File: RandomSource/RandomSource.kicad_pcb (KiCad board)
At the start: 2 copper layers, 154 x 128.5 mm, 74 parts, among them J1 Conn_01x20_Pin, J2 Conn_01x06_Pin, J6 Conn_01x20_Pin, Q1 BC547, Q2 BC547, Q3 BC547, Q4 BC557, Q5 MMBFJ113, Q6 2N7000, U1 TL074, U10 Aux_flush, U11 Aux_flush, U13 Aux_flush, U14 Aux_flush, U2 Aux_flush, U3 Switch, U4 TL074, U5 Switch, U6 Aux_flush, U7 Switch, U8 Switch, U9 Aux_flush

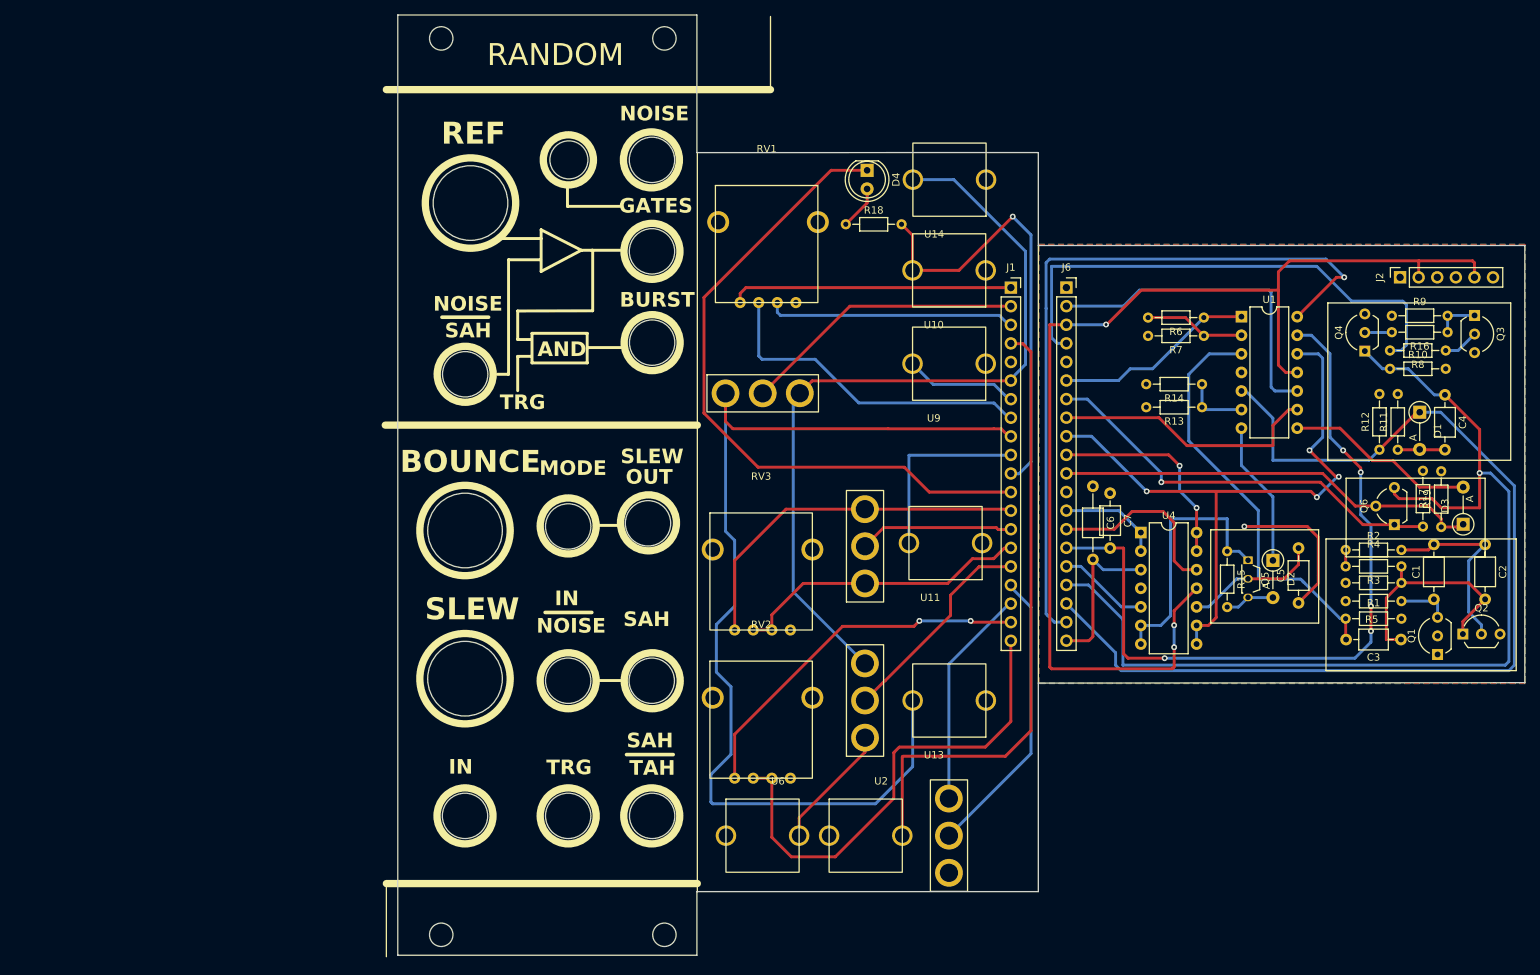
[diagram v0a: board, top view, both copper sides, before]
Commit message: Add files via upload
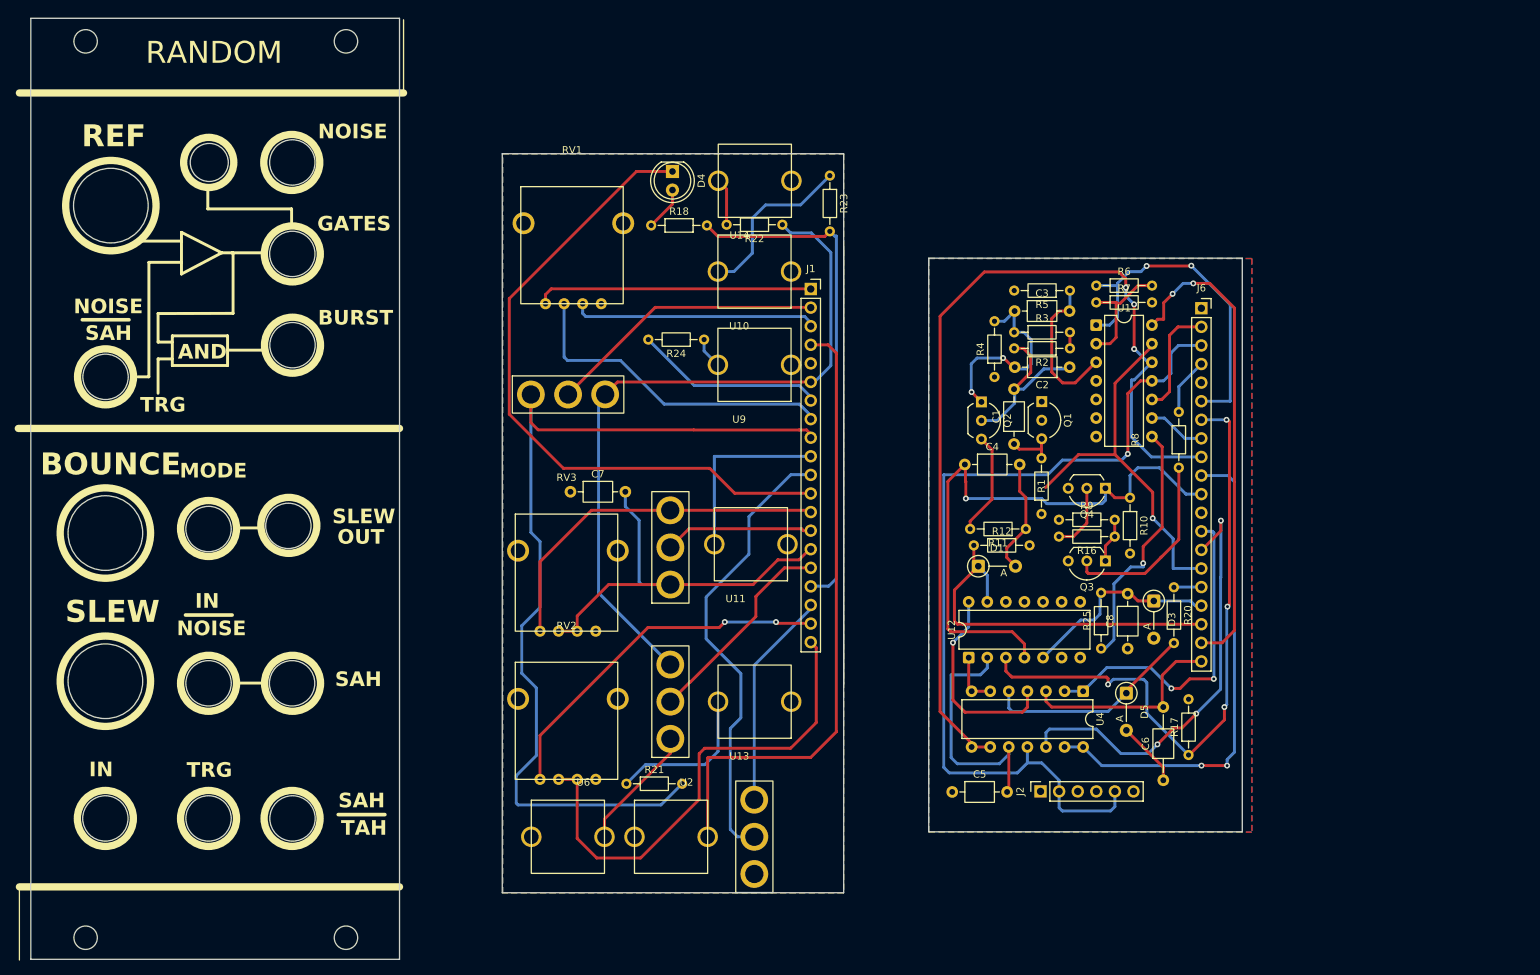
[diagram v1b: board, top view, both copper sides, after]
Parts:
- removed D2: D, Diode_THT:D_A-405_P5.08mm_Vertical_AnodeUp
- removed Q5: MMBFJ113, Package_TO_SOT_THT:TO-92S_Wide
- removed Q6: 2N7000, Package_TO_SOT_THT:TO-92L_Wide
- removed R13: 1k, Resistor_THT:R_Axial_DIN0204_L3.6mm_D1.6mm_P7.62mm_Horizontal
- removed R14, R19: 100k, Resistor_THT:R_Axial_DIN0204_L3.6mm_D1.6mm_P7.62mm_Horizontal
- removed R15: 1M, Resistor_THT:R_Axial_DIN0204_L3.6mm_D1.6mm_P7.62mm_Horizontal
- added C8: 100n, Capacitor_THT:C_Axial_L3.8mm_D2.6mm_P7.50mm_Horizontal, F.Cu at (185.0, 115.1)
- added D5: D, Diode_THT:D_A-405_P5.08mm_Vertical_AnodeUp, F.Cu at (184.8, 121.2)
- added R20: 10k, Resistor_THT:R_Axial_DIN0204_L3.6mm_D1.6mm_P7.62mm_Horizontal, F.Cu at (191.3, 106.7)
- added R21: 1k, Resistor_THT:R_Axial_DIN0204_L3.6mm_D1.6mm_P7.62mm_Horizontal, F.Cu at (116.5, 133.6)
- added R22: 1k, Resistor_THT:R_Axial_DIN0204_L3.6mm_D1.6mm_P7.62mm_Horizontal, F.Cu at (137.8, 57.2)
- added R23: 1k, Resistor_THT:R_Axial_DIN0204_L3.6mm_D1.6mm_P7.62mm_Horizontal, F.Cu at (144.3, 50.4)
- added R24: 1k, Resistor_THT:R_Axial_DIN0204_L3.6mm_D1.6mm_P7.62mm_Horizontal, F.Cu at (127.1, 72.9)
- added R25: 1k, Resistor_THT:R_Axial_DIN0204_L3.6mm_D1.6mm_P7.62mm_Horizontal, F.Cu at (181.4, 115.1)
- added U12: CD4066BE, Package_DIP:DIP-14_W7.62mm, F.Cu at (163.3, 116.3)
- moved J2 85.7 mm to (173.1, 134.6)
- moved C7 73.8 mm to (108.9, 93.7), turned to 0 degrees
- moved Q2 73.0 mm to (165.0, 81.4), turned to -90 degrees
- moved C3 69.3 mm to (169.6, 69.0), turned to 0 degrees
- moved C4 66.3 mm to (162.8, 89.9), turned to 0 degrees
- moved Q1 64.2 mm to (173.3, 81.3), turned to -90 degrees
- moved D1 63.9 mm to (164.6, 103.8), turned to 0 degrees
- moved R3 61.8 mm to (169.5, 71.9), turned to 0 degrees
- moved C2 61.7 mm to (177.1, 76.6), turned to 180 degrees
- moved C1 61.2 mm to (169.5, 87.1)
- moved Q3 60.6 mm to (182.0, 103.1), turned to 180 degrees
- moved R5 58.6 mm to (177.1, 66.2), turned to 180 degrees
- moved R12 57.0 mm to (164.0, 101.0), turned to 0 degrees
- moved R4 55.6 mm to (166.8, 78.0), turned to 90 degrees
- moved C5 53.9 mm to (161.0, 134.7), turned to 0 degrees
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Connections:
- D3 pad 2: Net-(D3-A) -> GND
- J1 pad 11: COMPO -> GATE
- J1 pad 17: GATE -> COMPO
- J6 pad 11: COMPO -> GATE
- J6 pad 17: GATE -> COMPO
- U1 pad 5: PULS -> (no net)
- U1 pad 6: Net-(U1B--) -> (no net)
- U1 pad 7: Net-(D2-K) -> (no net)
- U1 pad 8: Net-(D3-A) -> Net-(R25-Pad1)
- U10 pad 1: COMPO -> Net-(R23-Pad1)
- U13 pad 1: SAH -> Net-(R21-Pad1)
- U14 pad 1: NOISE -> Net-(R22-Pad2)
- U4 pad 5: SHIN -> Net-(D5-K)
- U9 pad 1: BURST -> Net-(R24-Pad1)
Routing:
- net PULS: track 172.7 -> 81.3 mm
- net TRG: track 155.9 -> 92.9 mm
- net BURST: track 71.9 -> 113.1 mm, vias 1 -> 4
- net DLY: track 54.4 -> 93.0 mm
- net GATE: track 181.4 -> 143.6 mm
- net S1: track 152.1 -> 115.3 mm, vias 3 -> 4
- net Net-(U1A-+): track 57.6 -> 20.8 mm
- net BC2: track 145.3 -> 109.7 mm, vias 5 -> 1
- net Net-(R25-Pad1): track 0.00 -> 34.3 mm, vias 0 -> 1
- net -12V: track 190.8 -> 156.5 mm, vias 3 -> 1
- net BOUNCE: track 46.0 -> 80.1 mm, vias 0 -> 3
- net BC1: track 64.0 -> 95.2 mm, vias 0 -> 2
- net COMP: track 85.3 -> 54.9 mm
- net Net-(D5-K): track 0.00 -> 29.1 mm
- net THR: track 81.8 -> 52.9 mm
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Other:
- board size 154 x 128.5 mm -> 165.6 x 128.6 mm
